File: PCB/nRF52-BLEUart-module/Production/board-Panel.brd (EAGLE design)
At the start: 164.7 x 202.7 mm, 942 parts, among them J1 USB-A_PTH_MALE, J10 USB-A_PTH_MALE, J11 USB-A_PTH_MALE, J12 USB-A_PTH_MALE, J13 USB-A_PTH_MALE, J14 USB-A_PTH_MALE, J15 USB-A_PTH_MALE, J16 USB-A_PTH_MALE, J17 USB-A_PTH_MALE, J18 USB-A_PTH_MALE, J19 USB-A_PTH_MALE, J2 USB-A_PTH_MALE, J20 USB-A_PTH_MALE, J21 USB-A_PTH_MALE, J22 USB-A_PTH_MALE, J23 USB-A_PTH_MALE, J24 USB-A_PTH_MALE, J3 USB-A_PTH_MALE, J4 USB-A_PTH_MALE, J5 USB-A_PTH_MALE, J6 USB-A_PTH_MALE, J7 USB-A_PTH_MALE, J8 USB-A_PTH_MALE, J9 USB-A_PTH_MALE, U1 CH340E, U10 CH340E, U11 NRF52832, U12 CH340E, U13 NRF52832, U14 CH340E, U15 NRF52832, U16 CH340E, U17 NRF52832, U18 CH340E, U19 NRF52832, U2 NRF52832, U20 CH340E, U21 NRF52832, U22 CH340E, U23 NRF52832, U24 CH340E, U25 NRF52832, U26 CH340E, U27 NRF52832, U28 CH340E, U29 NRF52832, U3 NRF52832, U30 CH340E, U31 NRF52832, U32 CH340E, U33 NRF52832, U34 CH340E, U35 NRF52832, U36 CH340E, U37 NRF52832, U38 CH340E, U39 NRF52832, U4 CH340E, U40 CH340E, U41 NRF52832, U42 CH340E, U43 NRF52832, U44 CH340E, U45 NRF52832, U46 CH340E, U47 NRF52832, U48 CH340E, U5 NRF52832, U6 CH340E, U7 NRF52832, U8 CH340E, U9 NRF52832, Y1 32MHz_2016, Y10 32MHz_2016, Y11 32.768kHz, Y12 32MHz_2016, Y13 32.768kHz, Y14 32MHz_2016, Y15 32.768kHz, Y16 32MHz_2016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

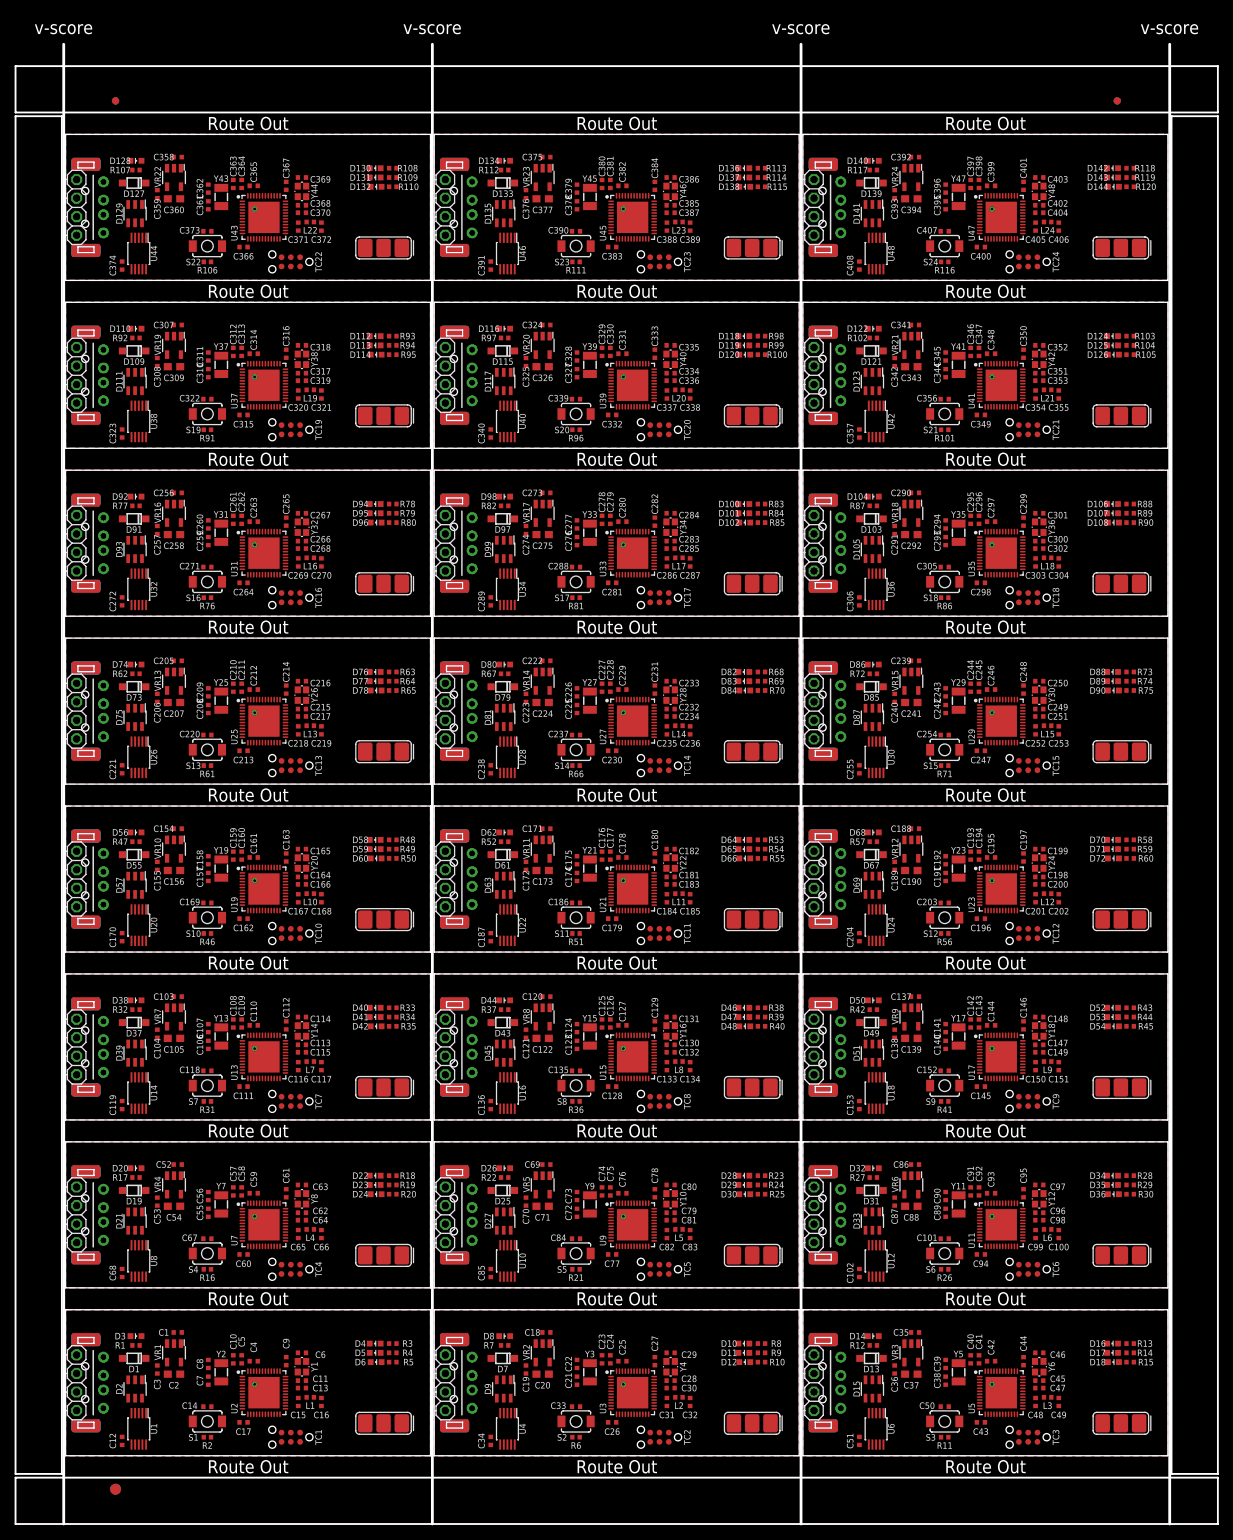
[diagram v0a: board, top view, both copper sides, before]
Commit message: final PCB for V1.0
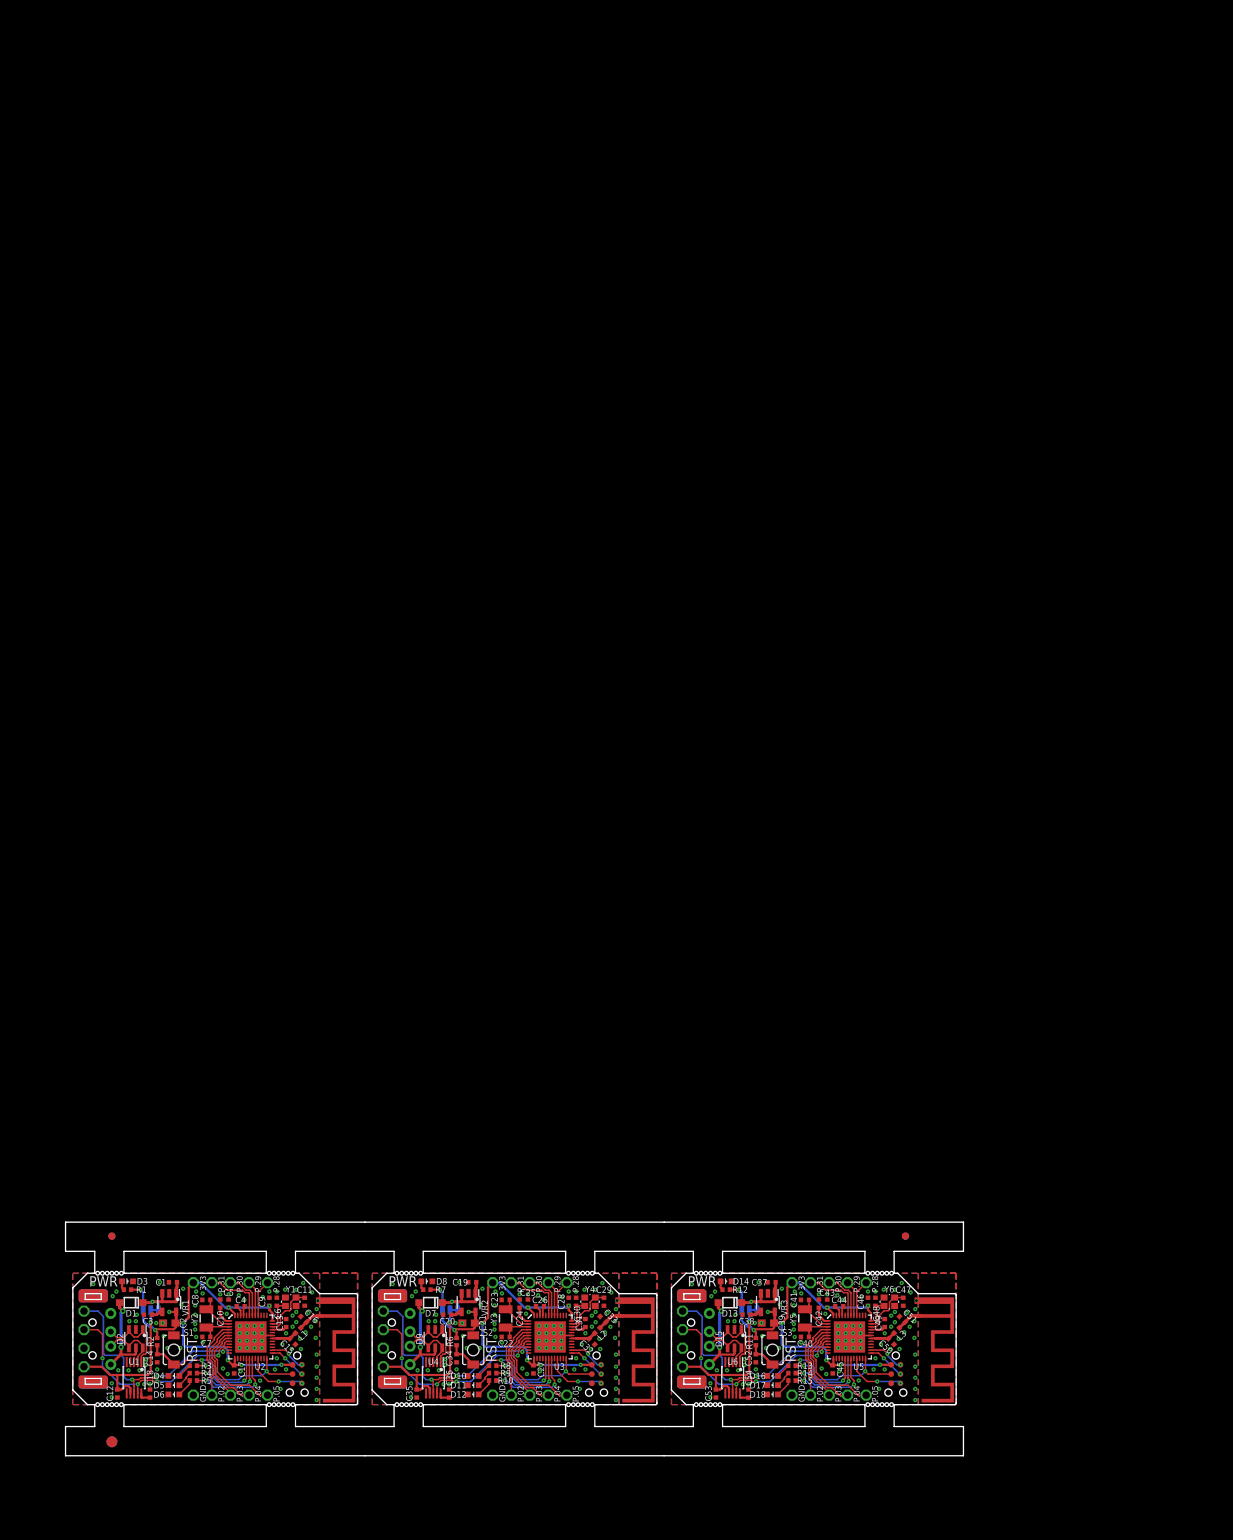
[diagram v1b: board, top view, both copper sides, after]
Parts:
- removed C100, C116, C117, C133, C134, C150, C151, C167, C168, C184, C185, C201, C202, C218, C219, C235, C236, C252, C253, C269, C270, C286, C287, C303, C304, C320, C321, C337, C338, C354, C355, C371, C372, C388, C389, C405, C406, C65, C66, C82, C83, C99: 0.8pF, angrypig7-RCL:C0402
- removed C101, C103, C118, C120, C135, C137, C152, C154, C169, C171, C186, C188, C203, C205, C220, C222, C237, C239, C254, C256, C271, C273, C288, C290, C305, C307, C322, C324, C339, C341, C356, C358, C373, C375, C390, C392, C407, C67, C69, C84, C86: 1uF, angrypig7-RCL:C0402
- removed C102, C104, C108, C110, C111, C112, C119, C121, C125, C127, C128, C129, C136, C138, C142, C144, C145, C146, C153, C155, C159, C161, C162, C163, C170, C172, C176, C178, C179, C180, C187, C189, C193, C195, C196, C197, C204, C206, C210, C212, C213, C214, C221, C223, C227, C229, C230, C231, C238, C240, C244, C246, C247, C248, C255, C257, C261, C263, C264, C265, C272, C274, C278, C280, C281, C282, C289, C291, C295, C297, C298, C299, C306, C308, C312, C314, C315, C316, C323, C325, C329, C331, C332, C333, C340, C342, C346, C348, C349, C350, C357, C359, C363, C365, C366, C367, C374, C376, C380, C382, C383, C384, C391, C393, C397, C399, C400, C401, C408, C57, C59, C60, C61, C68, C70, C74, C76, C77, C78, C85, C87, C91, C93, C94, C95: 100nF, angrypig7-RCL:C0402
- removed C105, C122, C139, C156, C173, C190, C207, C224, C241, C258, C275, C292, C309, C326, C343, C360, C377, C394, C71, C88: 2.2uF, angrypig7-RCL:C0603
- removed C106, C107, C113, C114, C123, C124, C130, C131, C140, C141, C147, C148, C157, C158, C164, C165, C174, C175, C181, C182, C191, C192, C198, C199, C208, C209, C215, C216, C225, C226, C232, C233, C242, C243, C249, C250, C259, C260, C266, C267, C276, C277, C283, C284, C293, C294, C300, C301, C310, C311, C317, C318, C327, C328, C334, C335, C344, C345, C351, C352, C361, C362, C368, C369, C378, C379, C385, C386, C395, C396, C402, C403, C55, C56, C62, C63, C72, C73, C79, C80, C89, C90, C96, C97: 12pF, angrypig7-RCL:C0402
- removed C109, C126, C143, C160, C177, C194, C211, C228, C245, C262, C279, C296, C313, C330, C347, C364, C381, C398, C58, C75, C92: 4.7uF, angrypig7-RCL:C0402
- removed C115, C132, C149, C166, C183, C200, C217, C234, C251, C268, C285, C302, C319, C336, C353, C370, C387, C404, C64, C81, C98: 100pF, angrypig7-RCL:C0402
- removed D100, D101, D102, D104, D106, D107, D108, D110, D112, D113, D114, D116, D118, D119, D120, D122, D124, D125, D126, D128, D130, D131, D132, D134, D136, D137, D138, D140, D142, D143, D144, D20, D22, D23, D24, D26, D28, D29, D30, D32, D34, D35, D36, D38, D40, D41, D42, D44, D46, D47, D48, D50, D52, D53, D54, D56, D58, D59, D60, D62, D64, D65, D66, D68, D70, D71, D72, D74, D76, D77, D78, D80, D82, D83, D84, D86, D88, D89, D90, D92, D94, D95, D96, D98: 0603, angrypig7-Diodes:LED_0603
- removed D103, D109, D115, D121, D127, D133, D139, D19, D25, D31, D37, D43, D49, D55, D61, D67, D73, D79, D85, D91, D97: B5819W, angrypig7-Diodes:SOD-123
- removed D105, D111, D117, D123, D129, D135, D141, D21, D27, D33, D39, D45, D51, D57, D63, D69, D75, D81, D87, D93, D99: TVS, angrypig7-Diodes:SPT-23-6
- removed J10, J11, J12, J13, J14, J15, J16, J17, J18, J19, J20, J21, J22, J23, J24, J4, J5, J6, J7, J8, J9: USB-A_PTH_MALE, angrypig7-Connectors-USB:USB-A-H-RECT
- removed JP13, JP14, JP15, JP16, JP17, JP18, JP19, JP20, JP21, JP22, JP23, JP24: V G Rx Tx, angrypig7-Connectors-PinHeads:1X04/90
- removed L10, L11, L12, L13, L14, L15, L16, L17, L18, L19, L20, L21, L22, L23, L24, L4, L5, L6, L7, L8, L9: (no value), angrypig7-RCL:R0402
- removed R100, R101, R102, R103, R104, R105, R106, R107, R108, R109, R110, R111, R112, R113, R114, R115, R116, R117, R118, R119, R120, R16, R17, R18, R19, R20, R21, R22, R23, R24, R25, R26, R27, R28, R29, R30, R31, R32, R33, R34, R35, R36, R37, R38, R39, R40, R41, R42, R43, R44, R45, R46, R47, R48, R49, R50, R51, R52, R53, R54, R55, R56, R57, R58, R59, R60, R61, R62, R63, R64, R65, R66, R67, R68, R69, R70, R71, R72, R73, R74, R75, R76, R77, R78, R79, R80, R81, R82, R83, R84, R85, R86, R87, R88, R89, R90, R91, R92, R93, R94, R95, R96, R97, R98, R99: 10k, angrypig7-RCL:R0402
- removed S10, S11, S12, S13, S14, S15, S16, S17, S18, S19, S20, S21, S22, S23, S24, S4, S5, S6, S7, S8, S9: SPST-3x4mm, angrypig7-Switches:TACTILE_SWITCH_SMD_3.0X4.0MM
- removed TC10, TC11, TC12, TC13, TC14, TC15, TC16, TC17, TC18, TC19, TC20, TC21, TC22, TC23, TC24, TC4, TC5, TC6, TC7, TC8, TC9: TC2030-IDC-NL, angrypig7-Connectors-Programming:TC2030-IDC-NL
- removed TP1, TP10, TP11, TP12, TP13, TP14, TP15, TP16, TP17, TP18, TP19, TP2, TP20, TP21, TP22, TP23, TP24, TP3, TP4, TP5, TP6, TP7, TP8, TP9: TEST-POINT-3, angrypig7-Tests:PAD-3X-RECT-SILK
- removed U10, U12, U14, U16, U18, U20, U22, U24, U26, U28, U30, U32, U34, U36, U38, U40, U42, U44, U46, U48, U8: CH340E, angrypig7-IC:MSOP-10
- removed U11, U13, U15, U17, U19, U21, U23, U25, U27, U29, U31, U33, U35, U37, U39, U41, U43, U45, U47, U7, U9: NRF52832, angrypig7-IC-MCU:QFN40P600X600X90-49T450N
- removed VR10, VR11, VR12, VR13, VR14, VR15, VR16, VR17, VR18, VR19, VR20, VR21, VR22, VR23, VR24, VR4, VR5, VR6, VR7, VR8, VR9: AP2210K-3.3TRG, angrypig7-IC-Power:SOT-23-5
- removed Y10, Y12, Y14, Y16, Y18, Y20, Y22, Y24, Y26, Y28, Y30, Y32, Y34, Y36, Y38, Y40, Y42, Y44, Y46, Y48, Y8: 32MHz_2016, angrypig7-Clocks:CRYSTAL-SMD-2.0X1.6MM
- removed Y11, Y13, Y15, Y17, Y19, Y21, Y23, Y25, Y27, Y29, Y31, Y33, Y35, Y37, Y39, Y41, Y43, Y45, Y47, Y7, Y9: 32.768kHz, angrypig7-Clocks:CRYSTAL-SMD-3.2X1.5MM
- added U$1, U$2, U$3: ANT, angrypig7-Antennas:TI-AN043_LEFT
- C15, C16, C32: value 0.8pF -> DNP
- C18, C35: value 1uF -> 100nF
- C19, C34: value 100nF -> 1uF
- C20, C54: value 2.2uF -> 100nF; device angrypig7-RCL:C0603 -> angrypig7-RCL:C0402
- C21, C39: value 12pF -> 2.2uF; device angrypig7-RCL:C0402 -> angrypig7-RCL:C0603
- C23, C40: value 100nF -> 12pF
- C24: value 4.7uF -> 100nF
- C25, C43: value 100nF -> 4.7uF
- C28, C38, C45, C46: value 12pF -> 100nF
- C30, C47: value 100pF -> 12pF
- C31, C49: value 0.8pF -> 100pF
- C33, C50: value 1uF -> DNP
- C37: value 2.2uF -> 1uF; device angrypig7-RCL:C0603 -> angrypig7-RCL:C0402
- C41: value 4.7uF -> 12pF
- C48: value 0.8pF -> 12pF
- C51: value 100nF -> DNP
- D14, D3, D8: value 0603 -> PWR
- JP1, JP5, JP9: value V G Rx Tx -> V G Tx Rx; device angrypig7-Connectors-PinHeads:1X04/90 -> angrypig7-Connectors-PinHeads:1X04-NOSILK
- JP10, JP2, JP6: value V G Rx Tx -> 5V 3V3; device angrypig7-Connectors-PinHeads:1X04/90 -> angrypig7-Jumpers:SMT-JUMPER_3_1-NC_TRACE_NO-SILK
- JP11, JP12, JP3, JP4, JP7, JP8: value V G Rx Tx -> (none); device angrypig7-Connectors-PinHeads:1X04/90 -> angrypig7-Connectors-PinHeads:1X05-NOSILK
- L1, L2, L3: value (none) -> 0R
- R1, R12, R7: value 10k -> 15k
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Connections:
- net N$15 renamed USB_IN1
- net N$2 renamed USB_IN
- net N$29 renamed USB_IN2
- removed net 3V10: C156.1, C160.1, C162.1, C163.1, C170.1, JP10.1, R46.2, R47.2, R48.2, R49.2, R50.2, TC10.1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
- removed net 3V11: C173.1, C177.1, C179.1, C180.1, C187.1, JP11.1, R51.2, R52.2, R53.2, R54.2, R55.2, TC11.1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
- removed net 3V12: C190.1, C194.1, C196.1, C197.1, C204.1, JP12.1, R56.2, R57.2, R58.2, R59.2, R60.2, TC12.1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
- removed net 3V13: C207.1, C211.1, C213.1, C214.1, C221.1, JP13.1, R61.2, R62.2, R63.2, R64.2, R65.2, TC13.1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
- removed net 3V14: C224.1, C228.1, C230.1, C231.1, C238.1, JP14.1, R66.2, R67.2, R68.2, R69.2, R70.2, TC14.1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
- removed net 3V15: C241.1, C245.1, C247.1, C248.1, C255.1, JP15.1, R71.2, R72.2, R73.2, R74.2, R75.2, TC15.1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
- removed net 3V16: C258.1, C262.1, C264.1, C265.1, C272.1, JP16.1, R76.2, R77.2, R78.2, R79.2, R80.2, TC16.1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
- removed net 3V17: C275.1, C279.1, C281.1, C282.1, C289.1, JP17.1, R81.2, R82.2, R83.2, R84.2, R85.2, TC17.1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
- removed net 3V18: C292.1, C296.1, C298.1, C299.1, C306.1, JP18.1, R86.2, R87.2, R88.2, R89.2, R90.2, TC18.1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
- removed net 3V19: C309.1, C313.1, C315.1, C316.1, C323.1, JP19.1, R91.2, R92.2, R93.2, R94.2, R95.2, TC19.1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
- removed net 3V20: C326.1, C330.1, C332.1, C333.1, C340.1, JP20.1, R100.2, R96.2, R97.2, R98.2, R99.2, TC20.1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
- removed net 3V21: C343.1, C347.1, C349.1, C350.1, C357.1, JP21.1, R101.2, R102.2, R103.2, R104.2, R105.2, TC21.1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
- removed net 3V22: C360.1, C364.1, C366.1, C367.1, C374.1, JP22.1, R106.2, R107.2, R108.2, R109.2, R110.2, TC22.1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
- removed net 3V23: C377.1, C381.1, C383.1, C384.1, C391.1, JP23.1, R111.2, R112.2, R113.2, R114.2, R115.2, TC23.1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
- removed net 3V24: C394.1, C398.1, C400.1, C401.1, C408.1, JP24.1, R116.2, R117.2, R118.2, R119.2, R120.2, TC24.1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
- removed net 3V4: C54.1, C58.1, C60.1, C61.1, C68.1, JP4.1, R16.2, R17.2, R18.2, R19.2, R20.2, TC4.1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
- removed net 3V5: C71.1, C75.1, C77.1, C78.1, C85.1, JP5.1, R21.2, R22.2, R23.2, R24.2, R25.2, TC5.1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
- removed net 3V6: C102.1, C88.1, C92.1, C94.1, C95.1, JP6.1, R26.2, R27.2, R28.2, R29.2, R30.2, TC6.1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
- removed net 3V7: C105.1, C109.1, C111.1, C112.1, C119.1, JP7.1, R31.2, R32.2, R33.2, R34.2, R35.2, TC7.1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
- removed net 3V8: C122.1, C126.1, C128.1, C129.1, C136.1, JP8.1, R36.2, R37.2, R38.2, R39.2, R40.2, TC8.1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
- removed net 3V9: C139.1, C143.1, C145.1, C146.1, C153.1, JP9.1, R41.2, R42.2, R43.2, R44.2, R45.2, TC9.1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
- removed net 5V10: C171.1, D61.C, TP11.P$3, VR11.1, VR11.3
- removed net 5V11: C188.1, D67.C, TP12.P$3, VR12.1, VR12.3
- removed net 5V12: C205.1, D73.C, TP13.P$3, VR13.1, VR13.3
- removed net 5V13: C222.1, D79.C, TP14.P$3, VR14.1, VR14.3
- removed net 5V14: C239.1, D85.C, TP15.P$3, VR15.1, VR15.3
- removed net 5V15: C256.1, D91.C, TP16.P$3, VR16.1, VR16.3
- removed net 5V16: C273.1, D97.C, TP17.P$3, VR17.1, VR17.3
- removed net 5V17: C290.1, D103.C, TP18.P$3, VR18.1, VR18.3
- removed net 5V18: C307.1, D109.C, TP19.P$3, VR19.1, VR19.3
- removed net 5V19: C324.1, D115.C, TP20.P$3, VR20.1, VR20.3
- removed net 5V20: C341.1, D121.C, TP21.P$3, VR21.1, VR21.3
- removed net 5V21: C358.1, D127.C, TP22.P$3, VR22.1, VR22.3
- removed net 5V22: C375.1, D133.C, TP23.P$3, VR23.1, VR23.3
- removed net 5V23: C392.1, D139.C, TP24.P$3, VR24.1, VR24.3
- removed net 5V3: C52.1, D19.C, TP4.P$3, VR4.1, VR4.3
- removed net 5V4: C69.1, D25.C, TP5.P$3, VR5.1, VR5.3
- removed net 5V5: C86.1, D31.C, TP6.P$3, VR6.1, VR6.3
- removed net 5V6: C103.1, D37.C, TP7.P$3, VR7.1, VR7.3
- removed net 5V7: C120.1, D43.C, TP8.P$3, VR8.1, VR8.3
- removed net 5V8: C137.1, D49.C, TP9.P$3, VR9.1, VR9.3
- removed net 5V9: C154.1, D55.C, TP10.P$3, VR10.1, VR10.3
- removed net GND10: C171.2, C172.2, C173.2, C174.1, C175.1, C176.2, C177.2, C178.2, C179.2, C180.2, C181.2, C182.2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
- removed net GND11: C188.2, C189.2, C190.2, C191.1, C192.1, C193.2, C194.2, C195.2, C196.2, C197.2, C198.2, C199.2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
- removed net GND12: C205.2, C206.2, C207.2, C208.1, C209.1, C210.2, C211.2, C212.2, C213.2, C214.2, C215.2, C216.2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
- removed net GND13: C222.2, C223.2, C224.2, C225.1, C226.1, C227.2, C228.2, C229.2, C230.2, C231.2, C232.2, C233.2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
- removed net GND14: C239.2, C240.2, C241.2, C242.1, C243.1, C244.2, C245.2, C246.2, C247.2, C248.2, C249.2, C250.2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
- removed net GND15: C256.2, C257.2, C258.2, C259.1, C260.1, C261.2, C262.2, C263.2, C264.2, C265.2, C266.2, C267.2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
- removed net GND16: C273.2, C274.2, C275.2, C276.1, C277.1, C278.2, C279.2, C280.2, C281.2, C282.2, C283.2, C284.2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
- removed net GND17: C290.2, C291.2, C292.2, C293.1, C294.1, C295.2, C296.2, C297.2, C298.2, C299.2, C300.2, C301.2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
- removed net GND18: C307.2, C308.2, C309.2, C310.1, C311.1, C312.2, C313.2, C314.2, C315.2, C316.2, C317.2, C318.2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
- removed net GND19: C324.2, C325.2, C326.2, C327.1, C328.1, C329.2, C330.2, C331.2, C332.2, C333.2, C334.2, C335.2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
- removed net GND20: C341.2, C342.2, C343.2, C344.1, C345.1, C346.2, C347.2, C348.2, C349.2, C350.2, C351.2, C352.2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
- removed net GND21: C358.2, C359.2, C360.2, C361.1, C362.1, C363.2, C364.2, C365.2, C366.2, C367.2, C368.2, C369.2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
- removed net GND22: C375.2, C376.2, C377.2, C378.1, C379.1, C380.2, C381.2, C382.2, C383.2, C384.2, C385.2, C386.2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
- removed net GND23: C392.2, C393.2, C394.2, C395.1, C396.1, C397.2, C398.2, C399.2, C400.2, C401.2, C402.2, C403.2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
- removed net GND3: C52.2, C53.2, C54.2, C55.1, C56.1, C57.2, C58.2, C59.2, C60.2, C61.2, C62.2, C63.2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
- removed net GND4: C69.2, C70.2, C71.2, C72.1, C73.1, C74.2, C75.2, C76.2, C77.2, C78.2, C79.2, C80.2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
- removed net GND5: C100.2, C101.2, C102.2, C86.2, C87.2, C88.2, C89.1, C90.1, C91.2, C92.2, C93.2, C94.2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
- removed net GND6: C103.2, C104.2, C105.2, C106.1, C107.1, C108.2, C109.2, C110.2, C111.2, C112.2, C113.2, C114.2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
- removed net GND7: C120.2, C121.2, C122.2, C123.1, C124.1, C125.2, C126.2, C127.2, C128.2, C129.2, C130.2, C131.2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
- removed net GND8: C137.2, C138.2, C139.2, C140.1, C141.1, C142.2, C143.2, C144.2, C145.2, C146.2, C147.2, C148.2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
- removed net GND9: C154.2, C155.2, C156.2, C157.1, C158.1, C159.2, C160.2, C161.2, C162.2, C163.2, C164.2, C165.2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
- removed net N$100: C121.1, VR8.4
- removed net N$101: C124.2, U15.2, Y15.P$2
- removed net N$102: C123.2, U15.3, Y15.P$1
- removed net N$103: C125.1, U15.1
- removed net N$104: C127.1, U15.46
- removed net N$105: C131.1, U15.35, Y16.3
- removed net N$106: C130.1, U15.34, Y16.1
- removed net N$107: C132.1, U15.33
- removed net N$108: U15.32
- removed net N$109: D44.A, R37.1
- removed net N$110: D46.A, R38.1
- removed net N$111: D47.A, R39.1
- removed net N$112: D48.A, R40.1
- removed net N$113: D49.A, D51.5, J9.VBUS
- removed net N$114: C138.1, VR9.4
- removed net N$115: C141.2, U17.2, Y17.P$2
- removed net N$116: C140.2, U17.3, Y17.P$1
- removed net N$117: C142.1, U17.1
- removed net N$118: C144.1, U17.46
- removed net N$119: C148.1, U17.35, Y18.3
- removed net N$120: C147.1, U17.34, Y18.1
- removed net N$121: C149.1, U17.33
- removed net N$122: U17.32
- removed net N$123: D50.A, R42.1
- removed net N$124: D52.A, R43.1
- removed net N$125: D53.A, R44.1
- removed net N$126: D54.A, R45.1
- removed net N$127: D55.A, D57.5, J10.VBUS
- removed net N$128: C155.1, VR10.4
- removed net N$129: C158.2, U19.2, Y19.P$2
- removed net N$130: C157.2, U19.3, Y19.P$1
- removed net N$131: C159.1, U19.1
- removed net N$132: C161.1, U19.46
- removed net N$133: C165.1, U19.35, Y20.3
- removed net N$134: C164.1, U19.34, Y20.1
- removed net N$135: C166.1, U19.33
- removed net N$136: U19.32
- removed net N$137: D56.A, R47.1
- removed net N$138: D58.A, R48.1
- removed net N$139: D59.A, R49.1
- removed net N$140: D60.A, R50.1
- removed net N$141: D61.A, D63.5, J11.VBUS
- removed net N$142: C172.1, VR11.4
- removed net N$143: C175.2, U21.2, Y21.P$2
- removed net N$144: C174.2, U21.3, Y21.P$1
- removed net N$145: C176.1, U21.1
- removed net N$146: C178.1, U21.46
- removed net N$147: C182.1, U21.35, Y22.3
- removed net N$148: C181.1, U21.34, Y22.1
- removed net N$149: C183.1, U21.33
- removed net N$150: U21.32
- removed net N$151: D62.A, R52.1
- removed net N$152: D64.A, R53.1
- removed net N$153: D65.A, R54.1
- removed net N$154: D66.A, R55.1
- removed net N$155: D67.A, D69.5, J12.VBUS
- removed net N$156: C189.1, VR12.4
- removed net N$157: C192.2, U23.2, Y23.P$2
- removed net N$158: C191.2, U23.3, Y23.P$1
- removed net N$159: C193.1, U23.1
- removed net N$160: C195.1, U23.46
- removed net N$161: C199.1, U23.35, Y24.3
- removed net N$162: C198.1, U23.34, Y24.1
- removed net N$163: C200.1, U23.33
- removed net N$164: U23.32
- removed net N$165: D68.A, R57.1
- removed net N$166: D70.A, R58.1
- removed net N$167: D71.A, R59.1
- removed net N$168: D72.A, R60.1
- removed net N$169: D73.A, D75.5, J13.VBUS
- removed net N$170: C206.1, VR13.4
- removed net N$171: C209.2, U25.2, Y25.P$2
- removed net N$172: C208.2, U25.3, Y25.P$1
- removed net N$173: C210.1, U25.1
- removed net N$174: C212.1, U25.46
- removed net N$175: C216.1, U25.35, Y26.3
- removed net N$176: C215.1, U25.34, Y26.1
- removed net N$177: C217.1, U25.33
- removed net N$178: U25.32
- removed net N$179: D74.A, R62.1
- removed net N$180: D76.A, R63.1
- removed net N$181: D77.A, R64.1
- removed net N$182: D78.A, R65.1
- removed net N$183: D79.A, D81.5, J14.VBUS
- removed net N$184: C223.1, VR14.4
- removed net N$185: C226.2, U27.2, Y27.P$2
- removed net N$186: C225.2, U27.3, Y27.P$1
- removed net N$187: C227.1, U27.1
- removed net N$188: C229.1, U27.46
- removed net N$189: C233.1, U27.35, Y28.3
- removed net N$190: C232.1, U27.34, Y28.1
- removed net N$191: C234.1, U27.33
- removed net N$192: U27.32
- removed net N$193: D80.A, R67.1
- removed net N$194: D82.A, R68.1
- removed net N$195: D83.A, R69.1
- removed net N$196: D84.A, R70.1
- removed net N$197: D85.A, D87.5, J15.VBUS
- removed net N$198: C240.1, VR15.4
- removed net N$199: C243.2, U29.2, Y29.P$2
- removed net N$200: C242.2, U29.3, Y29.P$1
- removed net N$201: C244.1, U29.1
- removed net N$202: C246.1, U29.46
- removed net N$203: C250.1, U29.35, Y30.3
- removed net N$204: C249.1, U29.34, Y30.1
- removed net N$205: C251.1, U29.33
- removed net N$206: U29.32
- removed net N$207: D86.A, R72.1
- removed net N$208: D88.A, R73.1
- removed net N$209: D89.A, R74.1
- removed net N$210: D90.A, R75.1
- removed net N$211: D91.A, D93.5, J16.VBUS
- removed net N$212: C257.1, VR16.4
- removed net N$213: C260.2, U31.2, Y31.P$2
- removed net N$214: C259.2, U31.3, Y31.P$1
- removed net N$215: C261.1, U31.1
- removed net N$216: C263.1, U31.46
- removed net N$217: C267.1, U31.35, Y32.3
- removed net N$218: C266.1, U31.34, Y32.1
- removed net N$219: C268.1, U31.33
- removed net N$220: U31.32
- removed net N$221: D92.A, R77.1
- removed net N$222: D94.A, R78.1
- removed net N$223: D95.A, R79.1
- removed net N$224: D96.A, R80.1
- removed net N$225: D97.A, D99.5, J17.VBUS
- removed net N$226: C274.1, VR17.4
- removed net N$227: C277.2, U33.2, Y33.P$2
- removed net N$228: C276.2, U33.3, Y33.P$1
- removed net N$229: C278.1, U33.1
- removed net N$23 (its old number): C30.1, U3.33
- removed net N$230: C280.1, U33.46
- removed net N$231: C284.1, U33.35, Y34.3
- removed net N$232: C283.1, U33.34, Y34.1
- removed net N$233: C285.1, U33.33
- removed net N$234: U33.32
- removed net N$235: D98.A, R82.1
- removed net N$236: D100.A, R83.1
- removed net N$237: D101.A, R84.1
- removed net N$238: D102.A, R85.1
- removed net N$239: D103.A, D105.5, J18.VBUS
- removed net N$240: C291.1, VR18.4
- removed net N$241: C294.2, U35.2, Y35.P$2
- removed net N$242: C293.2, U35.3, Y35.P$1
- removed net N$243: C295.1, U35.1
- removed net N$244: C297.1, U35.46
- removed net N$245: C301.1, U35.35, Y36.3
- removed net N$246: C300.1, U35.34, Y36.1
- removed net N$247: C302.1, U35.33
- removed net N$248: U35.32
- removed net N$249: D104.A, R87.1
- removed net N$250: D106.A, R88.1
- removed net N$251: D107.A, R89.1
- removed net N$252: D108.A, R90.1
- removed net N$253: D109.A, D111.5, J19.VBUS
- removed net N$254: C308.1, VR19.4
- removed net N$255: C311.2, U37.2, Y37.P$2
- removed net N$256: C310.2, U37.3, Y37.P$1
- removed net N$257: C312.1, U37.1
- removed net N$258: C314.1, U37.46
- removed net N$259: C318.1, U37.35, Y38.3
- removed net N$260: C317.1, U37.34, Y38.1
- removed net N$261: C319.1, U37.33
- removed net N$262: U37.32
- removed net N$263: D110.A, R92.1
- removed net N$264: D112.A, R93.1
- removed net N$265: D113.A, R94.1
- removed net N$266: D114.A, R95.1
- removed net N$267: D115.A, D117.5, J20.VBUS
- removed net N$268: C325.1, VR20.4
- removed net N$269: C328.2, U39.2, Y39.P$2
- removed net N$270: C327.2, U39.3, Y39.P$1
- removed net N$271: C329.1, U39.1
- removed net N$272: C331.1, U39.46
- removed net N$273: C335.1, U39.35, Y40.3
- removed net N$274: C334.1, U39.34, Y40.1
- removed net N$275: C336.1, U39.33
- removed net N$276: U39.32
- removed net N$277: D116.A, R97.1
- removed net N$278: D118.A, R98.1
- removed net N$279: D119.A, R99.1
- removed net N$280: D120.A, R100.1
- removed net N$281: D121.A, D123.5, J21.VBUS
- removed net N$282: C342.1, VR21.4
- removed net N$283: C345.2, U41.2, Y41.P$2
- removed net N$284: C344.2, U41.3, Y41.P$1
- removed net N$285: C346.1, U41.1
- removed net N$286: C348.1, U41.46
- removed net N$287: C352.1, U41.35, Y42.3
- removed net N$288: C351.1, U41.34, Y42.1
- removed net N$289: C353.1, U41.33
- removed net N$290: U41.32
- removed net N$291: D122.A, R102.1
- removed net N$292: D124.A, R103.1
- removed net N$293: D125.A, R104.1
- removed net N$294: D126.A, R105.1
- removed net N$295: D127.A, D129.5, J22.VBUS
- removed net N$296: C359.1, VR22.4
- removed net N$297: C362.2, U43.2, Y43.P$2
- removed net N$298: C361.2, U43.3, Y43.P$1
- removed net N$299: C363.1, U43.1
- removed net N$300: C365.1, U43.46
- removed net N$301: C369.1, U43.35, Y44.3
- removed net N$302: C368.1, U43.34, Y44.1
- removed net N$303: C370.1, U43.33
- removed net N$304: U43.32
- removed net N$305: D128.A, R107.1
- removed net N$306: D130.A, R108.1
- removed net N$307: D131.A, R109.1
- removed net N$308: D132.A, R110.1
- removed net N$309: D133.A, D135.5, J23.VBUS
- removed net N$310: C376.1, VR23.4
- removed net N$311: C379.2, U45.2, Y45.P$2
- removed net N$312: C378.2, U45.3, Y45.P$1
- removed net N$313: C380.1, U45.1
- removed net N$314: C382.1, U45.46
- removed net N$315: C386.1, U45.35, Y46.3
- removed net N$316: C385.1, U45.34, Y46.1
- removed net N$317: C387.1, U45.33
- removed net N$318: U45.32
- removed net N$319: D134.A, R112.1
- removed net N$320: D136.A, R113.1
- removed net N$321: D137.A, R114.1
- removed net N$322: D138.A, R115.1
- removed net N$323: D139.A, D141.5, J24.VBUS
- removed net N$324: C393.1, VR24.4
- removed net N$325: C396.2, U47.2, Y47.P$2
- removed net N$326: C395.2, U47.3, Y47.P$1
- removed net N$327: C397.1, U47.1
- removed net N$328: C399.1, U47.46
- removed net N$329: C403.1, U47.35, Y48.3
- removed net N$330: C402.1, U47.34, Y48.1
- removed net N$331: C404.1, U47.33
- removed net N$332: U47.32
- removed net N$333: D140.A, R117.1
- removed net N$334: D142.A, R118.1
- removed net N$335: D143.A, R119.1
- removed net N$336: D144.A, R120.1
- removed net N$37 (its old number): C47.1, U5.33
- removed net N$43: D19.A, D21.5, J4.VBUS
- removed net N$44: C53.1, VR4.4
- removed net N$45: C56.2, U7.2, Y7.P$2
- removed net N$46: C55.2, U7.3, Y7.P$1
- removed net N$47: C57.1, U7.1
- removed net N$48: C59.1, U7.46
- removed net N$49: C63.1, U7.35, Y8.3
- removed net N$50: C62.1, U7.34, Y8.1
- removed net N$51: C64.1, U7.33
- removed net N$52: U7.32
- removed net N$53: D20.A, R17.1
- removed net N$54: D22.A, R18.1
- removed net N$55: D23.A, R19.1
- removed net N$56: D24.A, R20.1
- removed net N$57: D25.A, D27.5, J5.VBUS
- removed net N$58: C70.1, VR5.4
- removed net N$59: C73.2, U9.2, Y9.P$2
- removed net N$60: C72.2, U9.3, Y9.P$1
- removed net N$61: C74.1, U9.1
- removed net N$62: C76.1, U9.46
- removed net N$63: C80.1, U9.35, Y10.3
- removed net N$64: C79.1, U9.34, Y10.1
- removed net N$65: C81.1, U9.33
- removed net N$66: U9.32
- removed net N$67: D26.A, R22.1
- removed net N$68: D28.A, R23.1
- removed net N$69: D29.A, R24.1
- removed net N$70: D30.A, R25.1
- removed net N$71: D31.A, D33.5, J6.VBUS
- removed net N$72: C87.1, VR6.4
- removed net N$73: C90.2, U11.2, Y11.P$2
- removed net N$74: C89.2, U11.3, Y11.P$1
- removed net N$75: C91.1, U11.1
- removed net N$76: C93.1, U11.46
- removed net N$77: C97.1, U11.35, Y12.3
- removed net N$78: C96.1, U11.34, Y12.1
- removed net N$79: C98.1, U11.33
- removed net N$80: U11.32
- removed net N$81: D32.A, R27.1
- removed net N$82: D34.A, R28.1
- removed net N$83: D35.A, R29.1
- removed net N$84: D36.A, R30.1
- removed net N$85: D37.A, D39.5, J7.VBUS
- removed net N$86: C104.1, VR7.4
- removed net N$87: C107.2, U13.2, Y13.P$2
- removed net N$88: C106.2, U13.3, Y13.P$1
- removed net N$89: C108.1, U13.1
- removed net N$90: C110.1, U13.46
- removed net N$91: C114.1, U13.35, Y14.3
- removed net N$92: C113.1, U13.34, Y14.1
- removed net N$93: C115.1, U13.33
- removed net N$94: U13.32
- removed net N$95: D38.A, R32.1
- removed net N$96: D40.A, R33.1
- removed net N$97: D41.A, R34.1
- removed net N$98: D42.A, R35.1
- removed net N$99: D43.A, D45.5, J8.VBUS
- removed net NRST10: C186.1, R51.1, S11.2, TC11.3, U21.24
- removed net NRST11: C203.1, R56.1, S12.2, TC12.3, U23.24
- removed net NRST12: C220.1, R61.1, S13.2, TC13.3, U25.24
- removed net NRST13: C237.1, R66.1, S14.2, TC14.3, U27.24
- removed net NRST14: C254.1, R71.1, S15.2, TC15.3, U29.24
- removed net NRST15: C271.1, R76.1, S16.2, TC16.3, U31.24
- removed net NRST16: C288.1, R81.1, S17.2, TC17.3, U33.24
- removed net NRST17: C305.1, R86.1, S18.2, TC18.3, U35.24
- removed net NRST18: C322.1, R91.1, S19.2, TC19.3, U37.24
- removed net NRST19: C339.1, R96.1, S20.2, TC20.3, U39.24
- removed net NRST20: C356.1, R101.1, S21.2, TC21.3, U41.24
- removed net NRST21: C373.1, R106.1, S22.2, TC22.3, U43.24
- removed net NRST22: C390.1, R111.1, S23.2, TC23.3, U45.24
- removed net NRST23: C407.1, R116.1, S24.2, TC24.3, U47.24
- removed net NRST3: C67.1, R16.1, S4.2, TC4.3, U7.24
- removed net NRST4: C84.1, R21.1, S5.2, TC5.3, U9.24
- removed net NRST5: C101.1, R26.1, S6.2, TC6.3, U11.24
- removed net NRST6: C118.1, R31.1, S7.2, TC7.3, U13.24
- removed net NRST7: C135.1, R36.1, S8.2, TC8.3, U15.24
- removed net NRST8: C152.1, R41.1, S9.2, TC9.3, U17.24
- removed net NRST9: C169.1, R46.1, S10.2, TC10.3, U19.24
- removed net RF-10: C83.1, L5.2
- removed net RF-11: C99.1, L6.1, U11.30
- removed net RF-12: C100.1, L6.2
- removed net RF-13: C116.1, L7.1, U13.30
- removed net RF-14: C117.1, L7.2
- removed net RF-15: C133.1, L8.1, U15.30
- removed net RF-16: C134.1, L8.2
- removed net RF-17: C150.1, L9.1, U17.30
- removed net RF-18: C151.1, L9.2
- removed net RF-19: C167.1, L10.1, U19.30
- removed net RF-20: C168.1, L10.2
- removed net RF-21: C184.1, L11.1, U21.30
- removed net RF-22: C185.1, L11.2
- removed net RF-23: C201.1, L12.1, U23.30
- removed net RF-24: C202.1, L12.2
- removed net RF-25: C218.1, L13.1, U25.30
- removed net RF-26: C219.1, L13.2
- removed net RF-27: C235.1, L14.1, U27.30
- removed net RF-28: C236.1, L14.2
- removed net RF-29: C252.1, L15.1, U29.30
- removed net RF-30: C253.1, L15.2
- removed net RF-31: C269.1, L16.1, U31.30
- removed net RF-32: C270.1, L16.2
- removed net RF-33: C286.1, L17.1, U33.30
- removed net RF-34: C287.1, L17.2
- removed net RF-35: C303.1, L18.1, U35.30
- removed net RF-36: C304.1, L18.2
- removed net RF-37: C320.1, L19.1, U37.30
- removed net RF-38: C321.1, L19.2
- removed net RF-39: C337.1, L20.1, U39.30
- removed net RF-40: C338.1, L20.2
- removed net RF-41: C354.1, L21.1, U41.30
- removed net RF-42: C355.1, L21.2
- removed net RF-43: C371.1, L22.1, U43.30
- removed net RF-44: C372.1, L22.2
- removed net RF-45: C388.1, L23.1, U45.30
- removed net RF-46: C389.1, L23.2
- removed net RF-47: C405.1, L24.1, U47.30
- removed net RF-48: C406.1, L24.2
- removed net RF-7: C65.1, L4.1, U7.30
- removed net RF-8: C66.1, L4.2
- removed net RF-9: C82.1, L5.1, U9.30
- removed net SWDCLK10: TC11.4, U21.25
- removed net SWDCLK11: TC12.4, U23.25
- removed net SWDCLK12: TC13.4, U25.25
- removed net SWDCLK13: TC14.4, U27.25
- removed net SWDCLK14: TC15.4, U29.25
- removed net SWDCLK15: TC16.4, U31.25
- removed net SWDCLK16: TC17.4, U33.25
- removed net SWDCLK17: TC18.4, U35.25
- removed net SWDCLK18: TC19.4, U37.25
- removed net SWDCLK19: TC20.4, U39.25
- removed net SWDCLK20: TC21.4, U41.25
- removed net SWDCLK21: TC22.4, U43.25
- removed net SWDCLK22: TC23.4, U45.25
- removed net SWDCLK23: TC24.4, U47.25
- removed net SWDCLK3: TC4.4, U7.25
- removed net SWDCLK4: TC5.4, U9.25
- removed net SWDCLK5: TC6.4, U11.25
- removed net SWDCLK6: TC7.4, U13.25
- removed net SWDCLK7: TC8.4, U15.25
- removed net SWDCLK8: TC9.4, U17.25
- removed net SWDCLK9: TC10.4, U19.25
- removed net SWDIO10: TC11.2, U21.26
- removed net SWDIO11: TC12.2, U23.26
- removed net SWDIO12: TC13.2, U25.26
- removed net SWDIO13: TC14.2, U27.26
- removed net SWDIO14: TC15.2, U29.26
- removed net SWDIO15: TC16.2, U31.26
- removed net SWDIO16: TC17.2, U33.26
- removed net SWDIO17: TC18.2, U35.26
- removed net SWDIO18: TC19.2, U37.26
- removed net SWDIO19: TC20.2, U39.26
- removed net SWDIO20: TC21.2, U41.26
- removed net SWDIO21: TC22.2, U43.26
- removed net SWDIO22: TC23.2, U45.26
- removed net SWDIO23: TC24.2, U47.26
- removed net SWDIO3: TC4.2, U7.26
- removed net SWDIO4: TC5.2, U9.26
- removed net SWDIO5: TC6.2, U11.26
- removed net SWDIO6: TC7.2, U13.26
- removed net SWDIO7: TC8.2, U15.26
- removed net SWDIO8: TC9.2, U17.26
- removed net SWDIO9: TC10.2, U19.26
- removed net SWO10: TC11.6, U21.21
- removed net SWO11: TC12.6, U23.21
- removed net SWO12: TC13.6, U25.21
- removed net SWO13: TC14.6, U27.21
- removed net SWO14: TC15.6, U29.21
- removed net SWO15: TC16.6, U31.21
- removed net SWO16: TC17.6, U33.21
- removed net SWO17: TC18.6, U35.21
- removed net SWO18: TC19.6, U37.21
- removed net SWO19: TC20.6, U39.21
- removed net SWO20: TC21.6, U41.21
- removed net SWO21: TC22.6, U43.21
- removed net SWO22: TC23.6, U45.21
- removed net SWO23: TC24.6, U47.21
- removed net SWO3: TC4.6, U7.21
- removed net SWO4: TC5.6, U9.21
- removed net SWO5: TC6.6, U11.21
- removed net SWO6: TC7.6, U13.21
- removed net SWO7: TC8.6, U15.21
- removed net SWO8: TC9.6, U17.21
- removed net SWO9: TC10.6, U19.21
- removed net UART_RX10: JP11.4, U22.9
- removed net UART_RX11: JP12.4, U24.9
- removed net UART_RX12: JP13.4, U26.9
- removed net UART_RX13: JP14.4, U28.9
- removed net UART_RX14: JP15.4, U30.9
- removed net UART_RX15: JP16.4, U32.9
- removed net UART_RX16: JP17.4, U34.9
- removed net UART_RX17: JP18.4, U36.9
- removed net UART_RX18: JP19.4, U38.9
- removed net UART_RX19: JP20.4, U40.9
- removed net UART_RX20: JP21.4, U42.9
- removed net UART_RX21: JP22.4, U44.9
- removed net UART_RX22: JP23.4, U46.9
- removed net UART_RX23: JP24.4, U48.9
- removed net UART_RX3: JP4.4, U8.9
- removed net UART_RX4: JP5.4, U10.9
- removed net UART_RX5: JP6.4, U12.9
- removed net UART_RX6: JP7.4, U14.9
- removed net UART_RX7: JP8.4, U16.9
- removed net UART_RX8: JP9.4, U18.9
- removed net UART_RX9: JP10.4, U20.9
- removed net UART_TX10: JP11.3, U22.8
- removed net UART_TX11: JP12.3, U24.8
- removed net UART_TX12: JP13.3, U26.8
- removed net UART_TX13: JP14.3, U28.8
- removed net UART_TX14: JP15.3, U30.8
- removed net UART_TX15: JP16.3, U32.8
- removed net UART_TX16: JP17.3, U34.8
- removed net UART_TX17: JP18.3, U36.8
- removed net UART_TX18: JP19.3, U38.8
- removed net UART_TX19: JP20.3, U40.8
- removed net UART_TX20: JP21.3, U42.8
- removed net UART_TX21: JP22.3, U44.8
- removed net UART_TX22: JP23.3, U46.8
- removed net UART_TX23: JP24.3, U48.8
- removed net UART_TX3: JP4.3, U8.8
- removed net UART_TX4: JP5.3, U10.8
- removed net UART_TX5: JP6.3, U12.8
- removed net UART_TX6: JP7.3, U14.8
- removed net UART_TX7: JP8.3, U16.8
- removed net UART_TX8: JP9.3, U18.8
- removed net UART_TX9: JP10.3, U20.8
- removed net USB_N10: D63.4, D63.6, J11.D-, U22.2
- removed net USB_N11: D69.4, D69.6, J12.D-, U24.2
- removed net USB_N12: D75.4, D75.6, J13.D-, U26.2
- removed net USB_N13: D81.4, D81.6, J14.D-, U28.2
- removed net USB_N14: D87.4, D87.6, J15.D-, U30.2
- removed net USB_N15: D93.4, D93.6, J16.D-, U32.2
- removed net USB_N16: D99.4, D99.6, J17.D-, U34.2
- removed net USB_N17: D105.4, D105.6, J18.D-, U36.2
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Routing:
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- added copper zone on layer 1, net GND-CUTOUT
- added copper zone on layer 1, net GND-CUTOUT1
- added copper zone on layer 16, net GND-CUTOUT2
- added copper zone on layer 16, net GND-CUTOUT3
- added copper zone on layer 1, net GND-CUTOUT4
- added copper zone on layer 16, net GND-CUTOUT5
- removed copper zone on layer 1, net GND10
- removed copper zone on layer 16, net GND10
- removed copper zone on layer 1, net GND11
- removed copper zone on layer 16, net GND11
- removed copper zone on layer 1, net GND12
- removed copper zone on layer 16, net GND12
- removed copper zone on layer 1, net GND13
- removed copper zone on layer 16, net GND13
- removed copper zone on layer 1, net GND14
- removed copper zone on layer 16, net GND14
- removed copper zone on layer 1, net GND15
- removed copper zone on layer 16, net GND15
- removed copper zone on layer 1, net GND16
- removed copper zone on layer 16, net GND16
- removed copper zone on layer 1, net GND17
- removed copper zone on layer 16, net GND17
- removed copper zone on layer 1, net GND18
- removed copper zone on layer 16, net GND18
- removed copper zone on layer 1, net GND19
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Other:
- board size 164.7 x 202.7 mm -> 123 x 32 mm
- board text added: "3V3 P.31 P.30 P.29 P.28"
- board text added: "GND P.02 P.03 P.04 P.05"
- board text added: "RST"
- board text removed: "Route Out"
- board text removed: "v-score"
